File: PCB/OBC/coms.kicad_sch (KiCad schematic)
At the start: 25 parts, among them U2 STM32F405RGTx

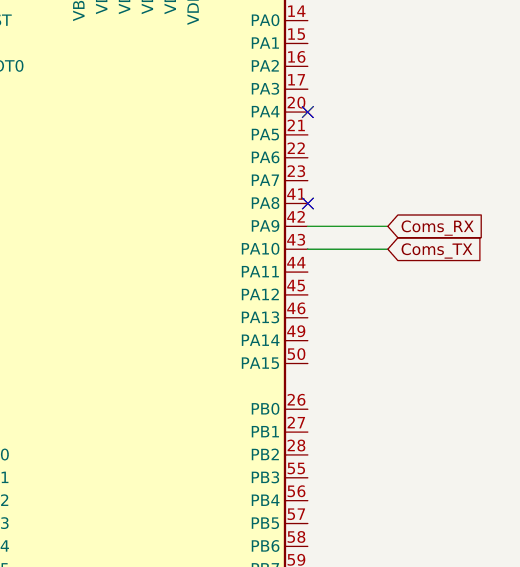
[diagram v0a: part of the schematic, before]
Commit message: minors changes
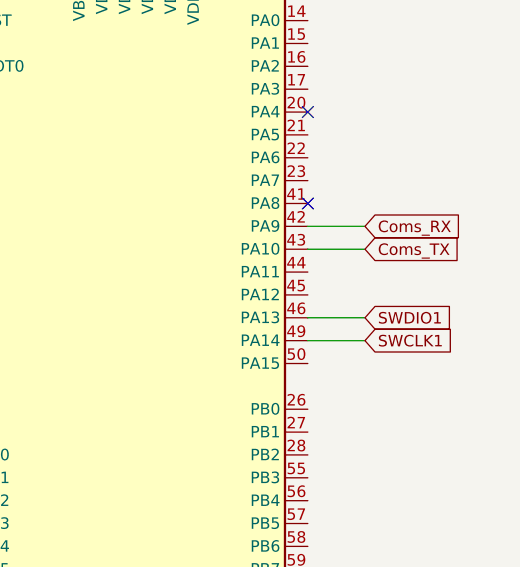
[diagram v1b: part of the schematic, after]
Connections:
- net SWDIO1: now reaches U2.46 (PA13)
- net SWCLK1: now reaches U2.49 (PA14)
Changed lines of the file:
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@@
 	(wire
 		(pts
-			(xy 137.16 71.12) (xy 146.05 71.12)
+			(xy 137.16 71.12) (xy 143.51 71.12)
 		)
 		(stroke
@@
 	(wire
 		(pts
-			(xy 137.16 73.66) (xy 146.05 73.66)
+			(xy 137.16 73.66) (xy 143.51 73.66)
 		)
 		(stroke
@@
 	(wire
 		(pts
+			(xy 137.16 81.28) (xy 143.51 81.28)
+		)
+		(stroke
+			(width 0)
+			(type default)
+		)
+	)
+	(wire
+		(pts
 			(xy 116.84 139.7) (xy 116.84 137.16)
 		)
@@
 		(pts
 			(xy 119.38 139.7) (xy 116.84 139.7)
+		)
+		(stroke
+			(width 0)
+			(type default)
+		)
+	)
+	(wire
+		(pts
+			(xy 137.16 83.82) (xy 143.51 83.82)
 		)
 		(stroke
@@
 		)
 	)
+	(global_label "SWCLK1"
+		(shape input)
+		(at 143.51 83.82 0)
+		(fields_autoplaced yes)
+		(effects
+			(font
+				(size 1.27 1.27)
+			)
+			(justify left)
+		)
+		(property "Intersheetrefs" "${INTERSHEET_REFS}"
+			(at 153.9337 83.82 0)
+			(effects
+				(font
+					(size 1.27 1.27)
+				)
+				(justify left)
+				(hide yes)
+			)
+		)
+	)
 	(global_label "Coms_TX"
 		(shape input)
-		(at 146.05 73.66 0)
+		(at 143.51 73.66 0)
 		(fields_autoplaced yes)
 		(effects
@@
 		)
 		(property "Intersheetrefs" "${INTERSHEET_REFS}"
-			(at 157.3203 73.66 0)
+			(at 154.7803 73.66 0)
 			(effects
 				(font
@@
 		)
 	)
+	(global_label "SWDIO1"
+		(shape input)
+		(at 143.51 81.28 0)
+		(fields_autoplaced yes)
+		(effects
+			(font
+				(size 1.27 1.27)
+			)
+			(justify left)
+		)
+		(property "Intersheetrefs" "${INTERSHEET_REFS}"
+			(at 153.5709 81.28 0)
+			(effects
+				(font
+					(size 1.27 1.27)
+				)
+				(justify left)
+				(hide yes)
+			)
+		)
+	)
 	(global_label "Coms_RX"
 		(shape input)
-		(at 146.05 71.12 0)
+		(at 143.51 71.12 0)
 		(fields_autoplaced yes)
 		(effects
@@
 		)
 		(property "Intersheetrefs" "${INTERSHEET_REFS}"
-			(at 157.6227 71.12 0)
+			(at 155.0827 71.12 0)
 			(effects
 				(font
